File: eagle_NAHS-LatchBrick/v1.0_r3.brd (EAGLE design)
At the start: 45.5 x 70.3 mm, 41 parts, among them IC1 ESP12S, IC2 ATTINY212-SSNR, IC3 TP4056, IC4 DW01A, J1 10118194-0001LF, J2 BRICK-INTERF-V3_B-SIDE, Q1 8205A

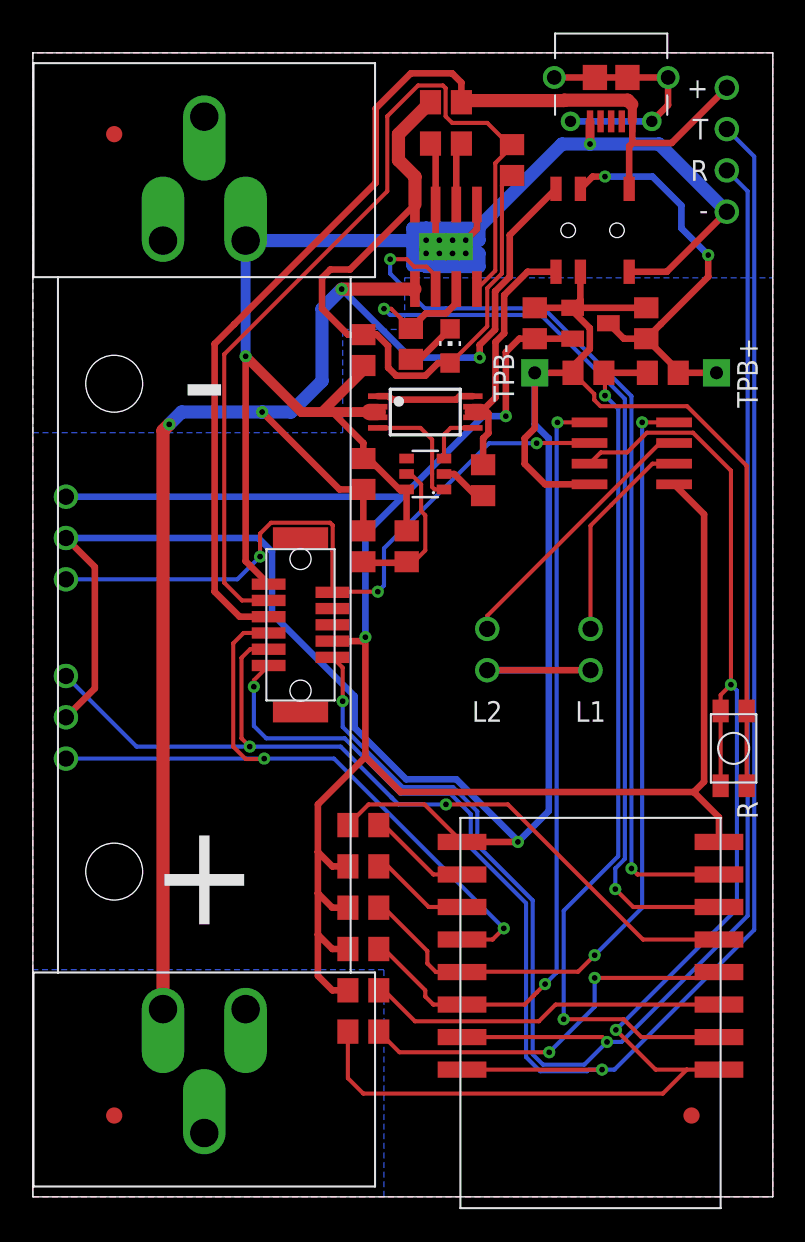
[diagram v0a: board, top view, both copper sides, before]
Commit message: v1.0 R3 Board done
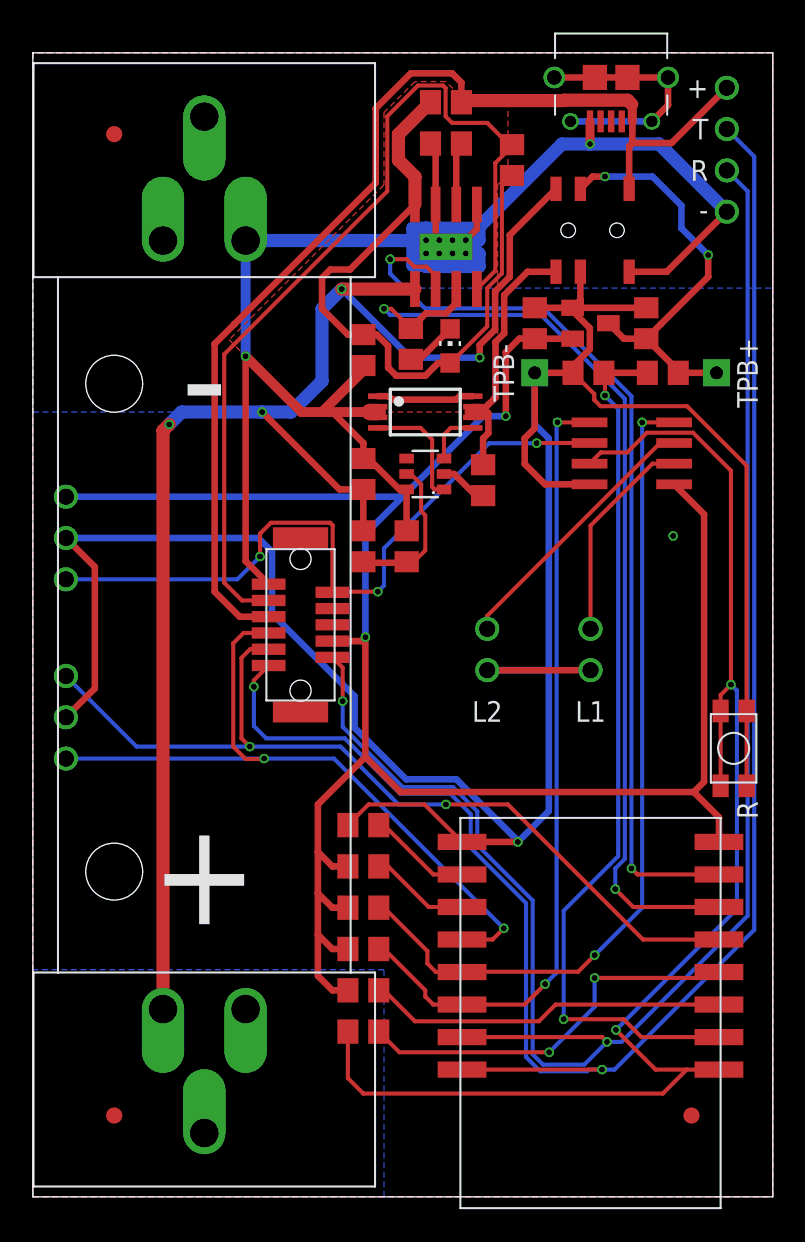
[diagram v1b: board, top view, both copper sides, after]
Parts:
- removed R15: 10k, rcl:R0805
- removed R16: 590k, rcl:R0805
- removed R17: 2.7M, rcl:R0805
- added R3, R4, R5: 1k, rcl:R0805
- R10, R11: value 3.9k -> 10k
- R13: value 10k -> 590k
- R14: value 10k -> 2.7M
- R6: value 1k -> 1.74k
- R7, R8: value 1k -> 3.9k
- R9: value 1.74k -> 10k
- moved R9 52.3 mm to (20.3, 12.7)
- moved R12 51.9 mm to (29.5, 63.8), turned to 90 degrees
- moved R7 34.8 mm to (20.3, 17.8), turned to 0 degrees
- moved R13 33.4 mm to (34.2, 50.7), turned to 180 degrees
- moved R14 33.4 mm to (38.7, 50.7), turned to 180 degrees
- moved R6 20.8 mm to (25.4, 64.8), turned to 0 degrees
- moved R11 7.62 mm to (20.3, 22.9)
- moved R8 5.08 mm to (20.3, 15.2), turned to 0 degrees
- moved R10 2.54 mm to (20.3, 20.3)
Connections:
- net +3V3: now also R7.1, R8.1, R9.1; no longer R11.1, R12.1, R13.1
- net A0: now also R13.1, R14.2; no longer R16.1, R17.2
- net BAT-: now also R3.1; no longer R6.1
- net BOOT1: now also R10.2; no longer R13.2
- net BOOT2: now also R11.2; no longer R14.2
- net CD: now also R12.2; no longer R15.2
- net CHRG: now also R4.2; no longer R7.2
- net EN: now also R9.2; no longer R12.2
- net GND: now also R11.1, R13.2; no longer R14.1, R16.2
- net IN-: now also R6.1; no longer R9.1
- net N$1: now also R12.1; no longer R15.1
- net N$2: now also R6.2; no longer R9.2
- net N$3: now also R3.2; no longer R6.2
- net N$7: now also R4.1; no longer R7.1
- net RST: now also R5.2; no longer R8.2
- net SCL: now also R8.2; no longer R11.2
- net SDA: now also R7.2; no longer R10.2
- net SEL+: now also R14.1; no longer R17.1
- net WAKE: now also R5.1; no longer R8.1
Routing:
- net GND: vias 1 -> 2
- added copper zone on layer 1, net N$1
